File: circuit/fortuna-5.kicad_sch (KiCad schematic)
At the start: 18 parts, among them J1 Debug, J8 USB-C Power, SW1 SW_Push, SW4 CLOCK, U1 ATmega2560-16C, U2 Z80CPU, U3 AS6C4008-55PCN, U4 74HC04, U5 74LS32, U6 74HC00

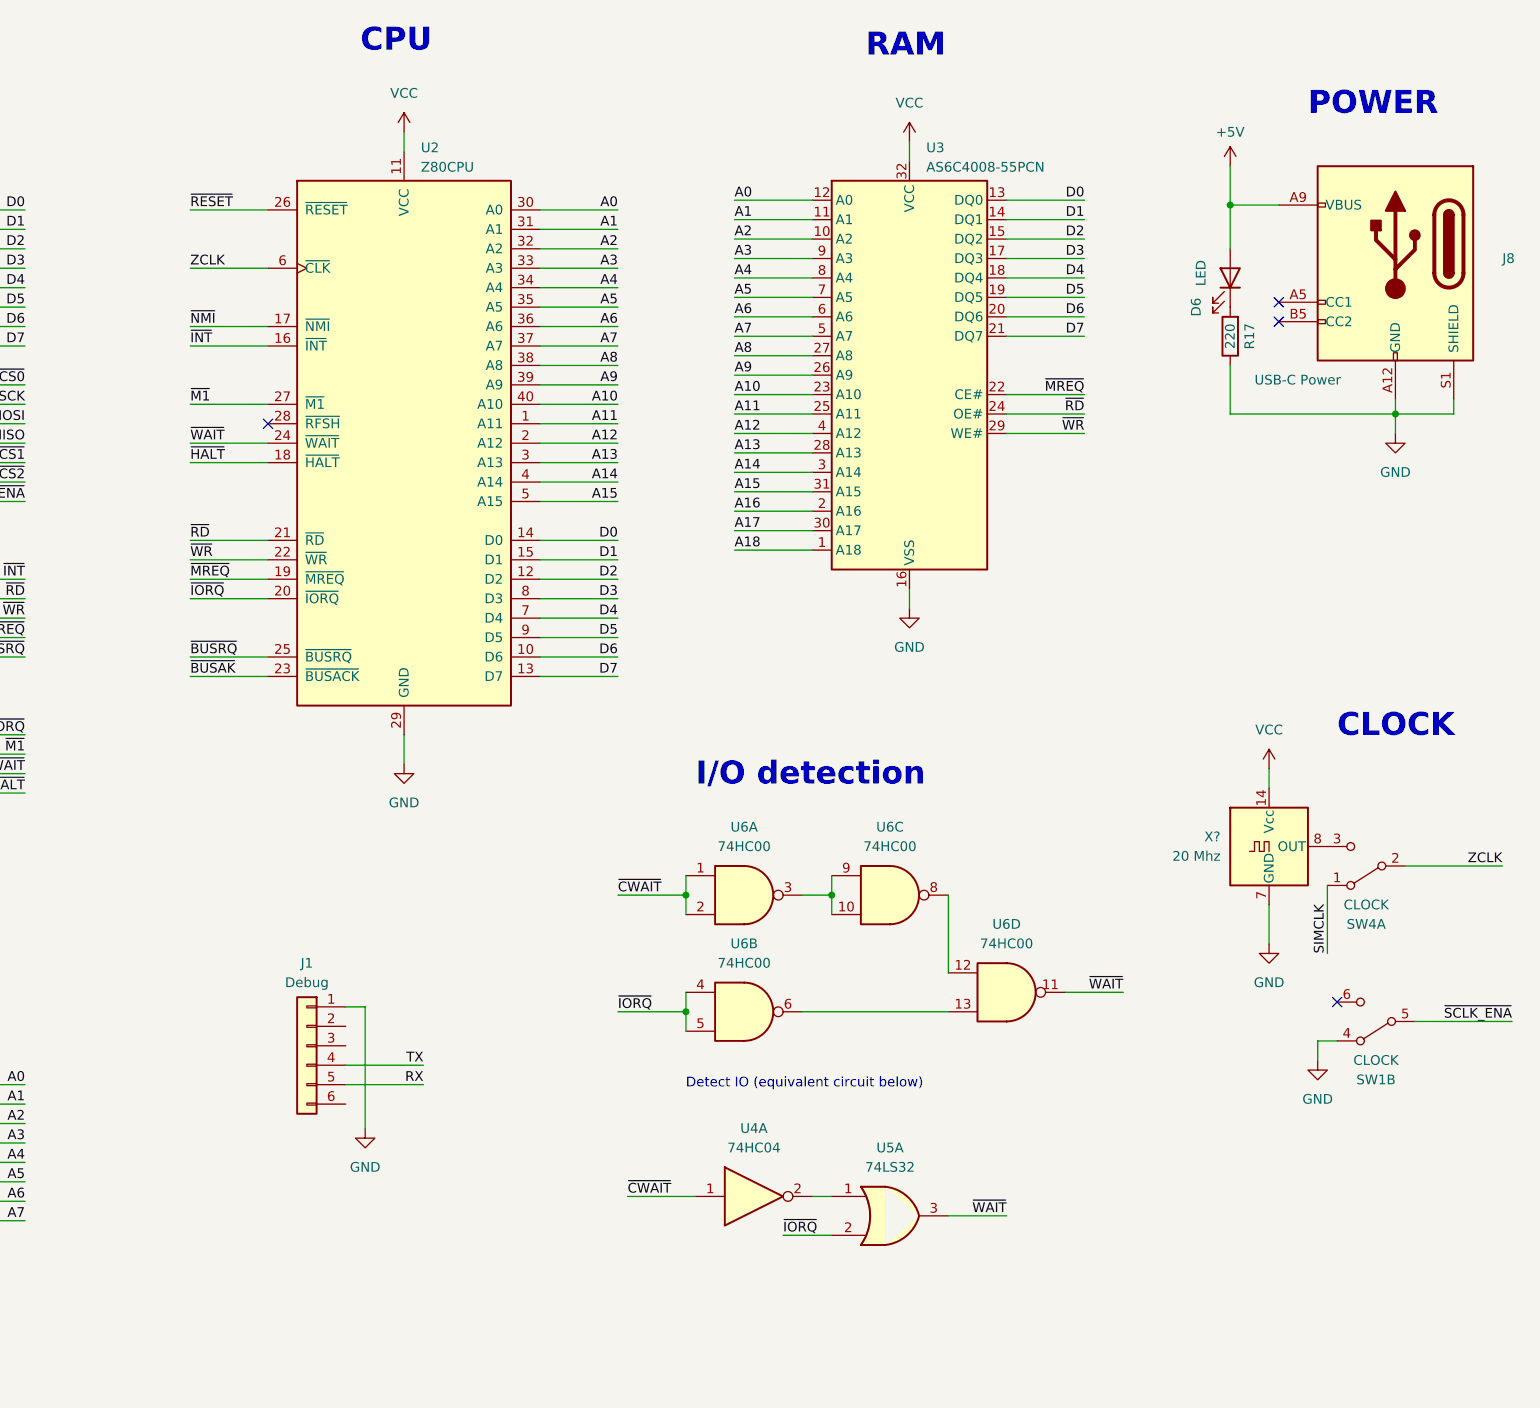
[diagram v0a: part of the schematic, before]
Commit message: .
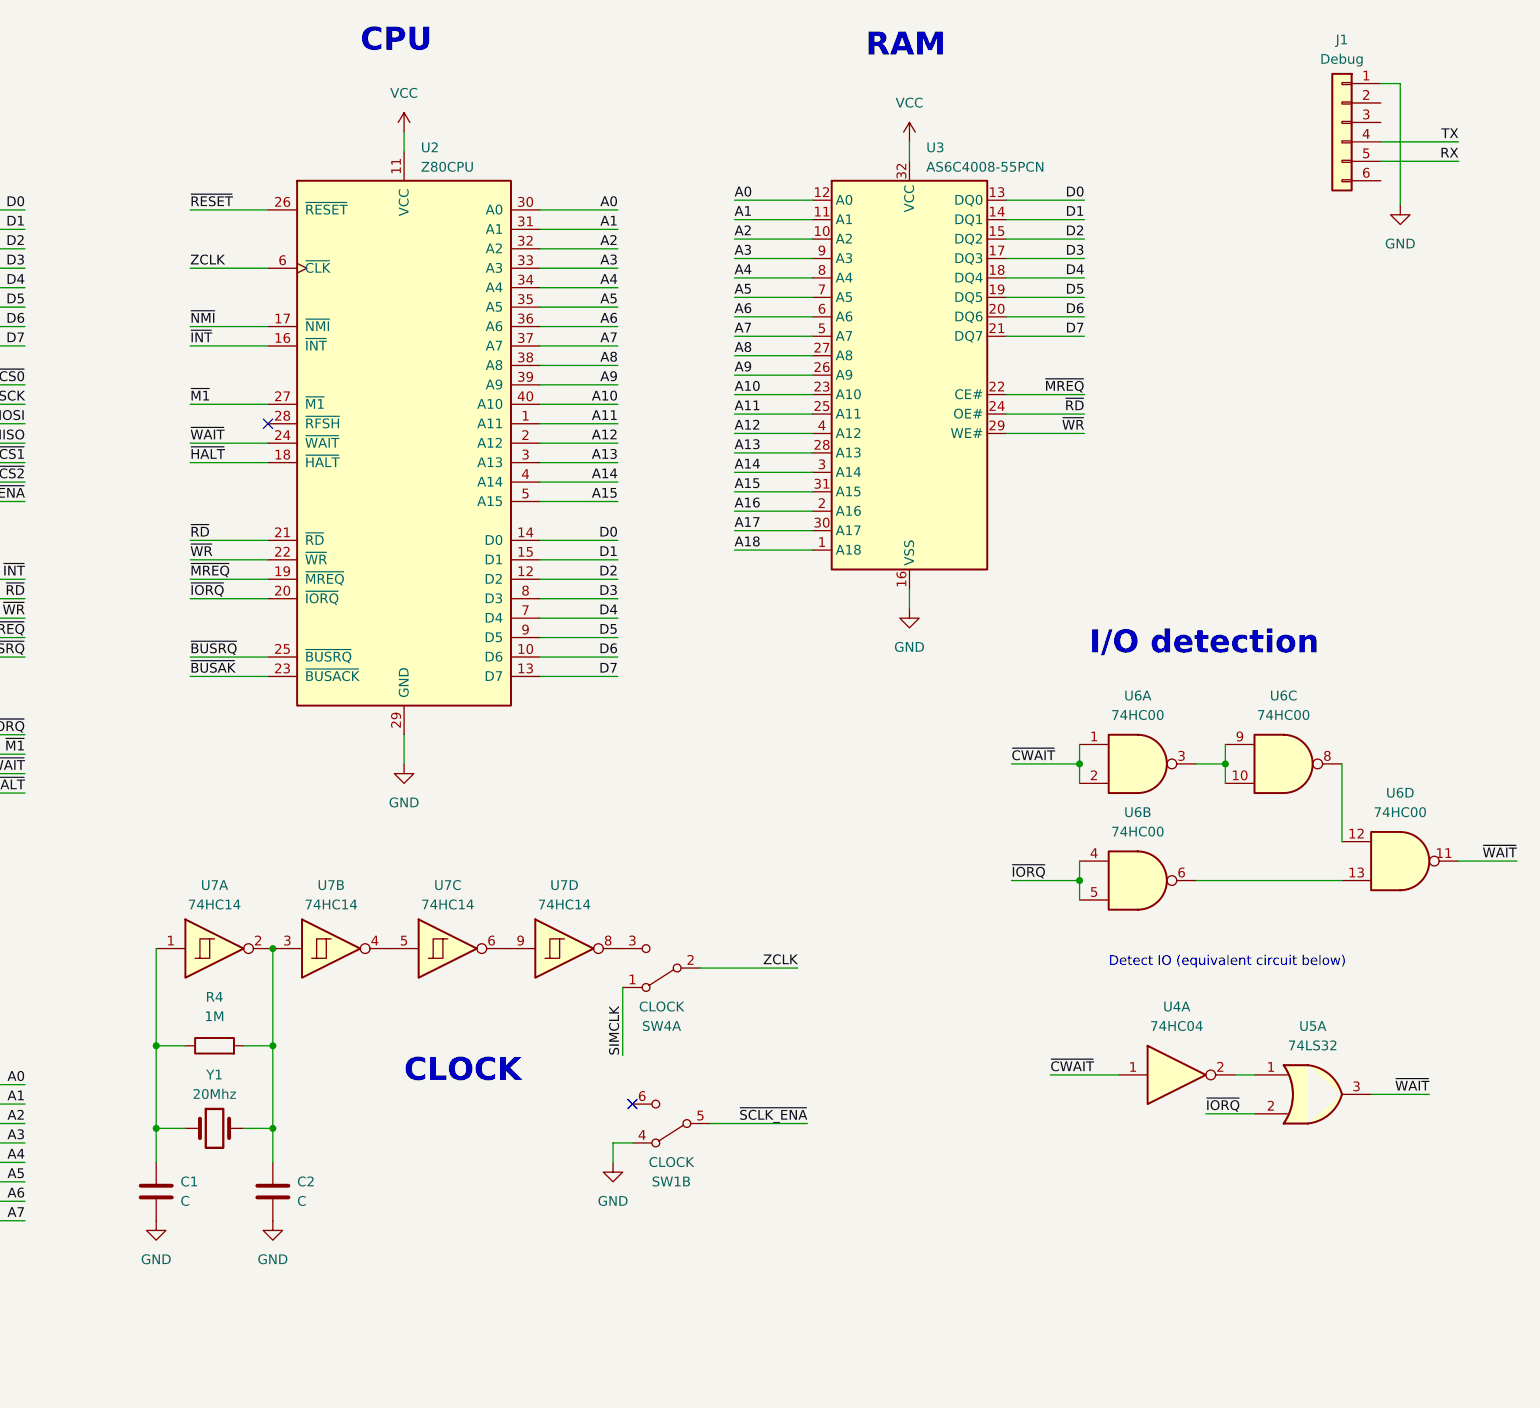
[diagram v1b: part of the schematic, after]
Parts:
- removed D6: LED, symbol Device:LED
- removed J8: USB-C Power, symbol Connector:USB_C_Receptacle_PowerOnly_6P
- removed R17: 220, symbol Device:R
- removed X?: 20 Mhz, Oscillator:Oscillator_DIP-14, symbol Oscillator:ACO-xxxMHz
- added C1, C2: C, symbol Device:C
- added R4: 1M, symbol Device:R
- added U7: 74HC14, symbol 74xx:74HC14
- added Y1: 20Mhz, symbol Device:Crystal
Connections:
- net GND: now also C1.2, C2.2
- net at SW4.3 (C): now also U7.8
- new net: U7.4, U7.5
- new net: U7.6, U7.9
- new net: C2.1, R4.2, U7.2, U7.3, Y1.2
- new net: C1.1, R4.1, U7.1, Y1.1
- no-connect marks 27 -> 25
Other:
- note removed: "POWER"
- moved on the sheet: J1, SW1B, SW4A, U4A, U5A, U6A, U6B, U6C, U6D
